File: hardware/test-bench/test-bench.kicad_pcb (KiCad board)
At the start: 2 copper layers, 90 x 90 mm, 33 parts, among them J1 Conn_Mem_Ext, J2 Conn_Reg, J3 SWD, J4 Conn_Mem, J5 FTDI, J6 Conn_Power, SW1 SW_Push_4pin, SW2 SW_Push_4pin, U1 STM32G030F6, U2 MCP23S17_SS, U3 MCP23S17_SS, U4 MCP23S17_SS, U5 MCP23S17_SS, U6 MIC5504-3.3YM5

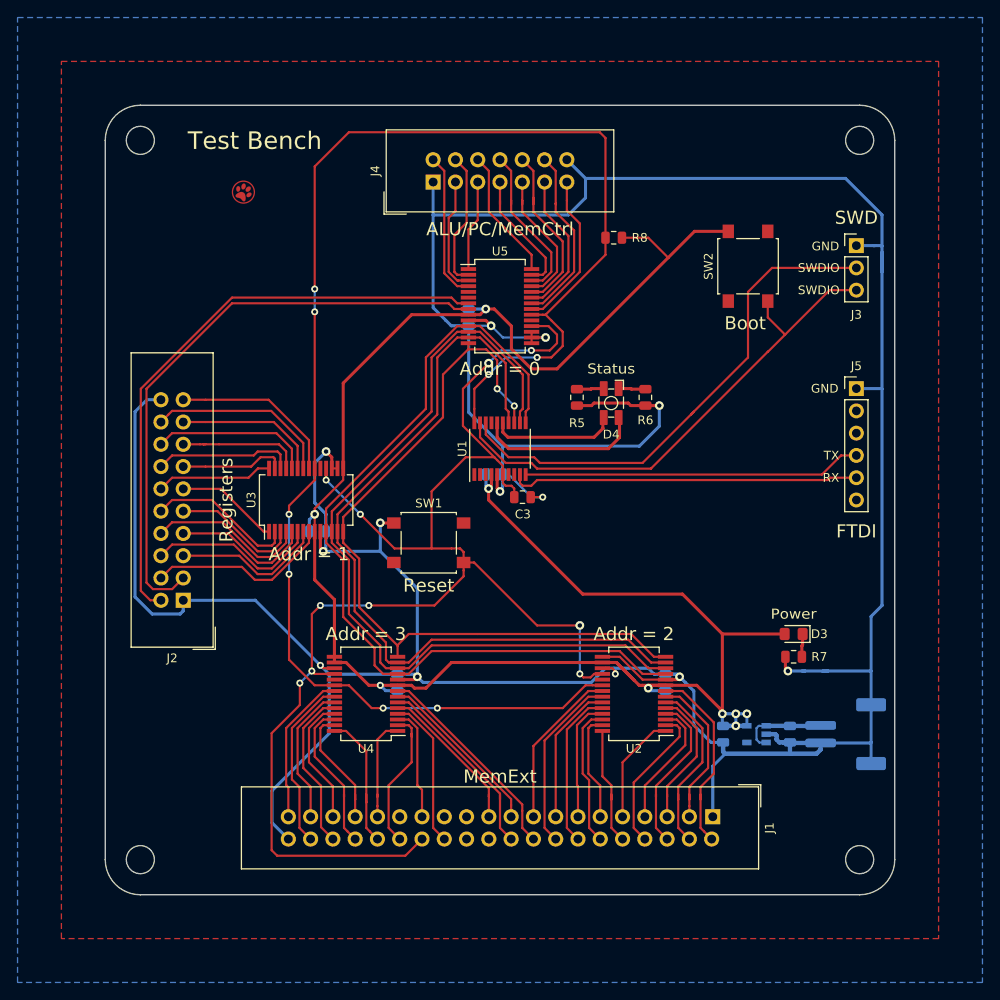
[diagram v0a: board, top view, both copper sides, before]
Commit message: Unified footprints
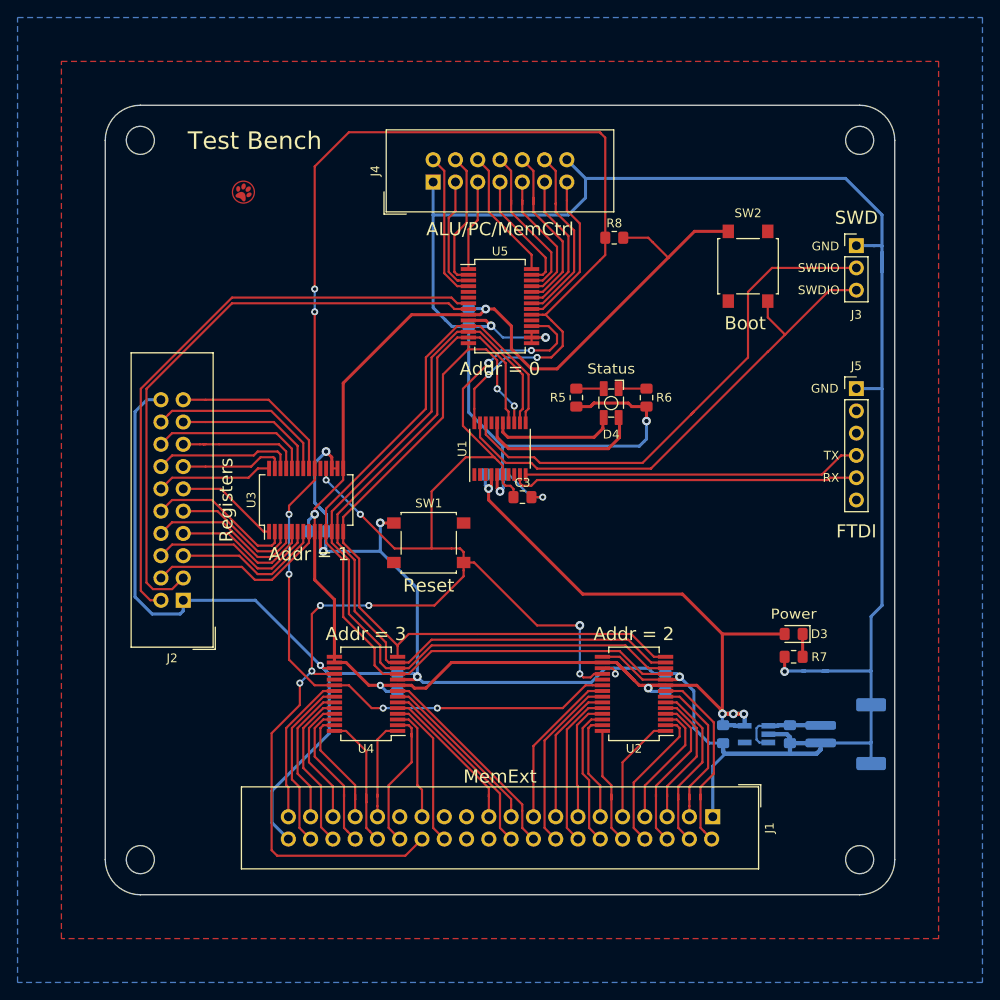
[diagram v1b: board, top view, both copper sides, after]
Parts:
- C1, C2, C3, C4, C5, C6, C7, C8: footprint Capacitor_SMD:C_0805_2012Metric -> Capacitor_SMD:C_0805_2012Metric_Pad1.15x1.40mm_HandSolder
- R5, R6, R7, R8: footprint Resistor_SMD:R_0805_2012Metric -> Resistor_SMD:R_0805_2012Metric_Pad1.15x1.40mm_HandSolder
- U6: footprint Package_TO_SOT_SMD:SOT-23-5 -> Package_TO_SOT_SMD:SOT-23-5_HandSoldering
- moved R6 0.13 mm to (178.7, 56.3)
- moved R5 0.08 mm to (170.7, 56.3)
- moved R8 0.06 mm to (175.0, 38.1)
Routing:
- net VCC: track 225.0 -> 225.6 mm, vias 9 -> 8
